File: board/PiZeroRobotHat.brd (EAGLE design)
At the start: 65 x 30 mm, 31 parts, among them IC1 TPS63061, IC2 MEGA8-AI, J1 AVRISP6_TP, Q1 CSTCR6M00G53Z, U1 DRV8835, U2 PCA9306, X1 1751248, X2 1751248, X3 1751248

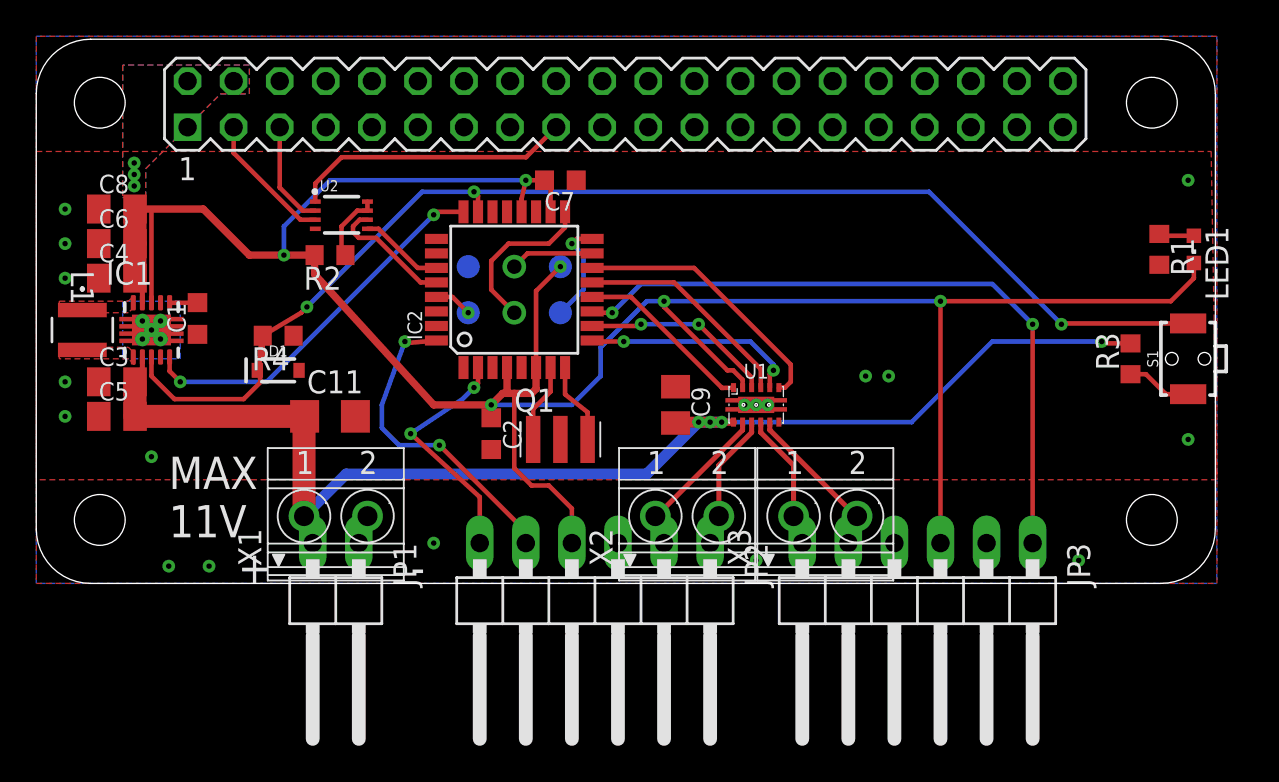
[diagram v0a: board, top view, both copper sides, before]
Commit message: board improvements
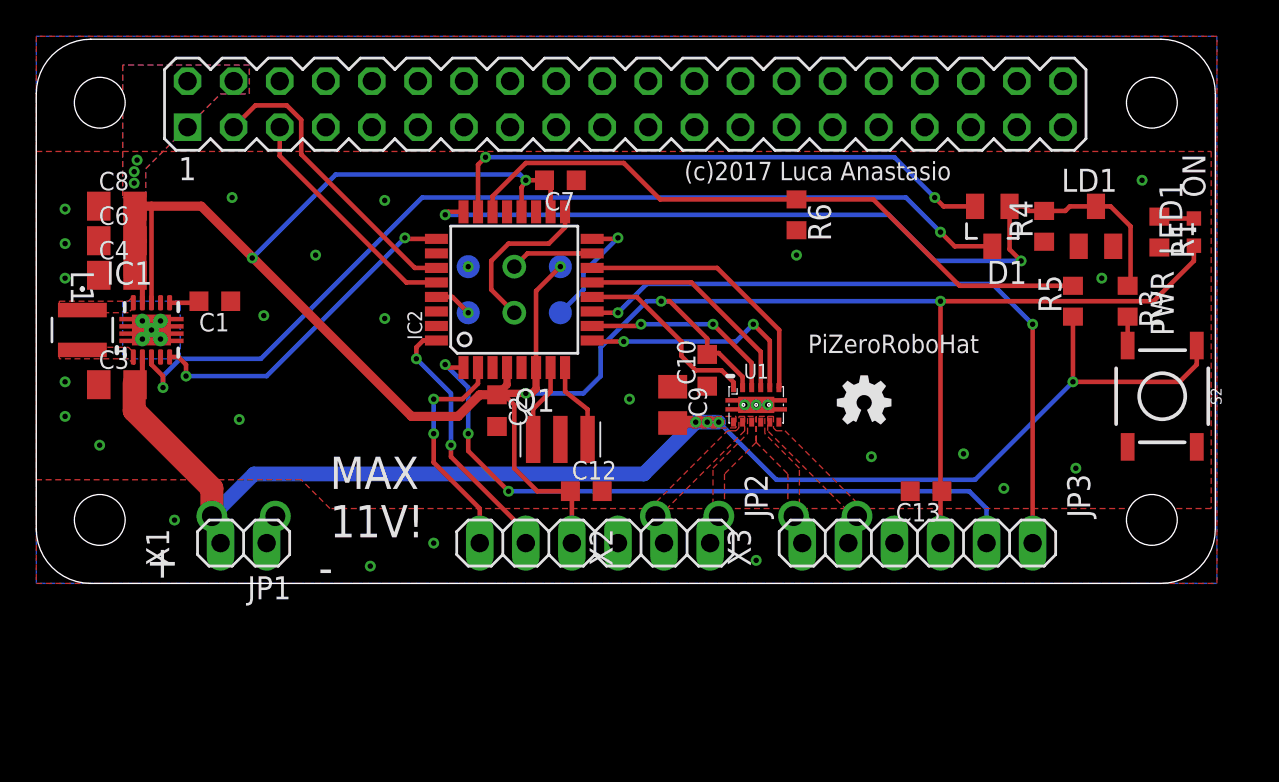
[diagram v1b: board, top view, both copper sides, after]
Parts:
- removed C11: 100uF, eagle-ltspice:C1206
- removed C5: 10uF, rcl:C0805K
- removed R2: 200K, resistor:R0603
- removed S1: MOMENTARY-SWITCH-SPST-SMD-RIGHT-ANGLE, SparkFun-Switches:TACTILE_SWITCH_SMD_RIGHT_ANGLE
- removed U2: PCA9306, SparkFun-IC-Comms:PCA9306DC
- added C10, C12, C13: 0.1uF, rcl:C0603K
- added LD1: PL006-WCR12, led:SOT23
- added R5: 470k, rcl:R0603
- added R6: 330k, rcl:R0603
- added S2: MOMENTARY-SWITCH-SPST-SMD-5.2-REDUNDANT, SparkFun-Switches:TACTILE_SWITCH_SMD_5.2MM
- D1: value 5.6V -> BAT54C; device SparkFun-DiscreteSemi:SOD-323 -> diode:SOT23
- JP1: device pinhead:1X02/90 -> pinhead:1X02
- JP2, JP3: device pinhead:1X06/90 -> pinhead:1X06
- R3: value 1M -> 10K
- R4: value 10M -> 1M
- moved R4 42.7 mm to (55.6, 19.7), turned to 90 degrees
- moved D1 40.2 mm to (52.7, 19.7), turned to 180 degrees
- moved JP1 6.35 mm to (11.4, 2.22)
- moved X1 5.08 mm to (11.4, 3.81)
- moved JP2 3.81 mm to (30.8, 2.22)
- moved JP3 3.81 mm to (48.6, 2.22)
- moved R3 3.18 mm to (60.2, 15.6), turned to 270 degrees
- moved C1 1.35 mm to (9.84, 15.6), turned to 180 degrees
- moved C2 1.31 mm to (25.4, 9.53)
- moved LED1 0.95 mm to (63.8, 19.4), turned to 0 degrees
- moved R1 0.95 mm to (61.9, 19.4)
- moved C3 0.16 mm to (4.45, 11.0)
- moved C8 0.16 mm to (4.45, 20.8)
- moved C4 0.16 mm to (4.45, 17.0)
- moved C6 0.16 mm to (4.45, 18.9)
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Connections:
- net N$10 renamed M1A
- net N$6 renamed M0A
- net N$8 renamed M1B
- net N$9 renamed M0B
- removed net 3.3V: U$1.17, U2.1
- removed net N$2: R2.1, U2.7, U2.8
- removed net SCL1: U$1.5, U2.2
- removed net SCL2: IC2.28, U2.6
- removed net SDA1: U$1.3, U2.3
- removed net SDA2: IC2.27, U2.5
- new net BUTTON: D1.1, IC2.24, LD1.3, R3.1, R4.2
- new net PS_ON: D1.2, IC2.23
- new net SCL: IC2.28, U$1.5
- new net SDA: IC2.27, U$1.3
- net 5V: now also C10.2, C12.1, C13.1, LED1.A; no longer LED1.C, R2.2
- net ENABLE: now also D1.3; no longer D1.C, IC2.23, R4.2, S1.2
- net GND: now also C10.1, C12.2, C13.2, LD1.1, R6.2; no longer C11.2, C5.1, D1.A, U2.4
- net N$1: now also R3.2, S2.3, S2.4; no longer R3.1, S1.1
- net N$7: now also LED1.C; no longer LED1.A
- net POWER_GOOD: now also IC2.25; no longer IC2.24
- net VBAT: now also R5.2, R6.1
- net VIN: now also R5.1, S2.1, S2.2; no longer C11.1, C5.2, R3.2
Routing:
- net BUTTON: track 0.00 -> 47.8 mm, vias 0 -> 2
- net ENC1_A: track 0.00 -> 38.2 mm, vias 0 -> 3
- net VBAT: track 0.00 -> 36.4 mm
- net PS_ON: track 0.00 -> 31.3 mm, vias 0 -> 2
- net ENABLE: track 71.8 -> 53.5 mm, vias 3 -> 2
- net SDA: track 0.00 -> 16.5 mm
- net 3.3V: track 15.6 -> 0.00 mm
- net SCL: track 0.00 -> 13.1 mm
- net VIN: track 71.1 -> 81.9 mm
- net SDA1: track 7.45 -> 0.00 mm
- net M1B: track 8.90 -> 1.69 mm
- net M0B: track 8.77 -> 1.56 mm
- net SCL2: track 7.01 -> 0.00 mm
- net M1A: track 7.62 -> 1.69 mm
- net M0A: track 7.62 -> 1.69 mm
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- added copper zone on layer 1, net M0A
- added copper zone on layer 1, net M0B
- added copper zone on layer 1, net M1A
- added copper zone on layer 1, net M1B
- added copper zone on layer 1, net VIN
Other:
- board text added: "(c)2017 Luca Anastasio"
- board text added: "/home/luca/Immagini/oshw.bmp"
- board text added: "MAX 11V!"
- board text added: "ON"
- board text added: "PWR"
- board text added: "PiZeroRoboHat"
- board text removed: "MAX 11V"

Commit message: board improvements
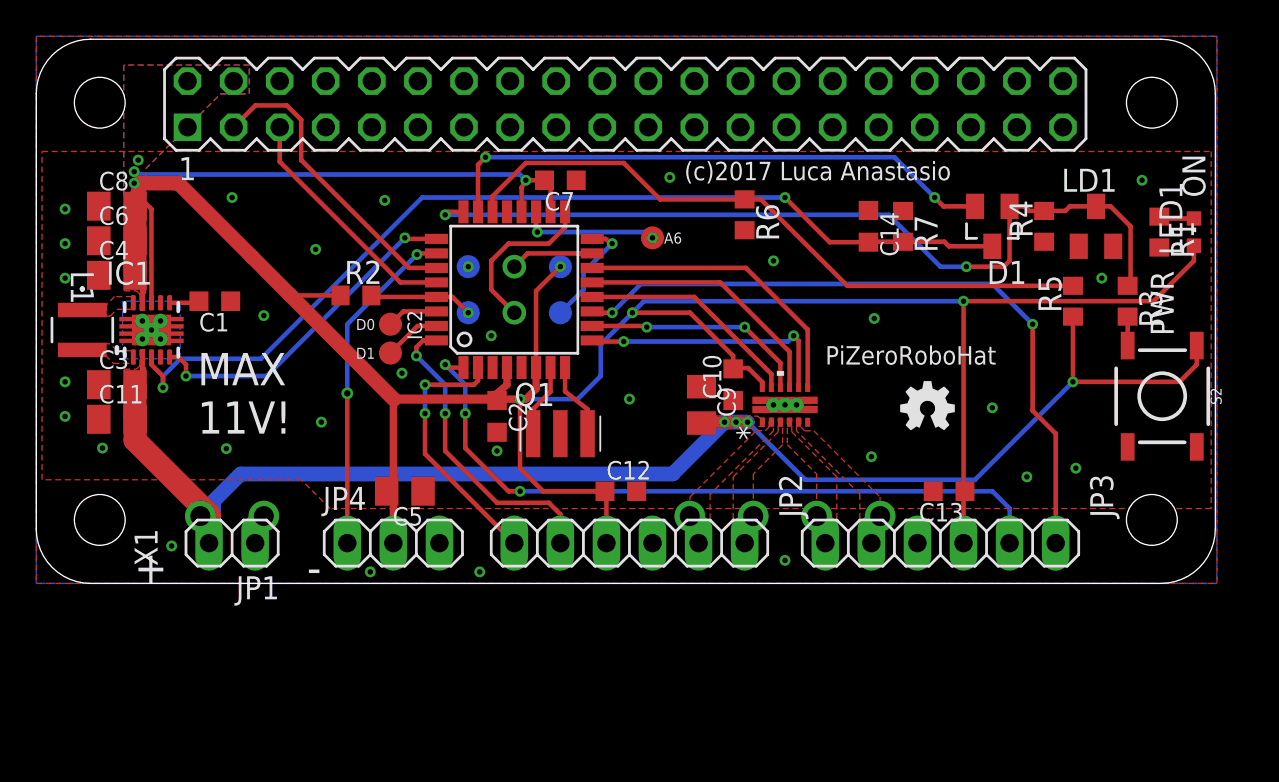
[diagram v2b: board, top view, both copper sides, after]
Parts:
- removed U1: DRV8835, bt_motordriver:WSON_2X3
- removed X2, X3: 1751248, con-phoenix-350:1751248
- added C11, C5: 10uF, rcl:C0805K
- added C14: 0.1uF, rcl:C0603K
- added JP4: (no value), pinhead:1X03
- added R2: 10K, resistor:R0603
- added R7: 1M, resistor:R0603
- added TP1, TP2, TP3: TEST-POINT3X5, SparkFun-Connectors:PAD.03X.05
- added U2: DRV8835DSSR, drv8835:DSS12_P9X2
- added X4: 1751264, con-phoenix-350:1751264
- moved R6 2.86 mm to (39.1, 20.3)
- moved C12 1.91 mm to (32.2, 5.08)
- moved JP2 1.91 mm to (32.7, 2.22)
- moved C10 1.63 mm to (38.4, 11.0)
- moved C9 1.59 mm to (36.7, 9.84)
- moved C13 1.27 mm to (50.3, 5.08)
- moved JP3 1.27 mm to (49.8, 2.22)
- moved JP1 0.63 mm to (10.8, 2.22)
- moved X1 0.63 mm to (10.8, 3.81)
- moved C2 0.32 mm to (25.4, 9.21)
- moved Q1 0.32 mm to (28.9, 8.26)
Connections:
- new net 0: IC2.30, TP1.P$1
- new net 1: IC2.31, TP2.P$1
- new net N$8: IC2.19, TP3.P$1
- new net SERVO: IC2.26, JP4.1
- net 5V: now also C5.2, JP4.2, R2.1, U2.12; no longer U1.11
- net ENABLE: now also C14.2, R7.2
- net EN_A: now also U2.9; no longer U1.9
- net EN_B: now also U2.7; no longer U1.7
- net GND: now also C11.1, C14.1, C5.1, JP4.3, R7.1, U2.13, U2.14, U2.15, U2.16, U2.17, U2.18, U2.6, U2.P$1, U2.P$2, U2.P$3; no longer U1.6, U1.PAD, U1.PAD1, U1.PAD2, U1.PAD3, U1.PAD4
- net M0A: now also U2.3, X4.2; no longer U1.3, X2.2
- net M0B: now also U2.2, X4.1; no longer U1.2, X2.1
- net M1A: now also U2.4, X4.3; no longer U1.4, X3.1
- net M1B: now also U2.5, X4.4; no longer U1.5, X3.2
- net MODE: now also U2.11; no longer U1.12
- net PH_A: now also U2.10; no longer U1.10
- net PH_B: now also U2.8; no longer U1.8
- net RST: now also R2.2
- net VIN: now also C11.2, U2.1; no longer U1.1
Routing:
- net 5V: track 143.7 -> 167.3 mm, vias 9 -> 8
- net SERVO: track 0.00 -> 18.6 mm, vias 0 -> 2
- net N$8: track 0.00 -> 7.63 mm, vias 0 -> 2
- net RST: track 2.11 -> 6.19 mm
- net 1: track 0.00 -> 3.15 mm
- net VIN: track 81.9 -> 85.0 mm
- net 0: track 0.00 -> 2.83 mm
- net ENC0_A: track 14.6 -> 17.0 mm
- net MODE: track 10.5 -> 12.4 mm
- net ENC0_B: track 12.7 -> 14.5 mm
- net EN_A: track 12.9 -> 14.4 mm
- net M0B: track 1.56 -> 0.00 mm
- net EN_B: track 14.9 -> 16.5 mm
- net PH_A: track 11.1 -> 12.6 mm
- net ENC1_A: track 38.2 -> 39.4 mm
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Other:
- board text added: "5V"
- board text added: "A"
- board text added: "A6"
- board text added: "B"
- board text added: "D0"
- board text added: "D1"
- board text added: "M+"
- board text added: "M-"
- board text added: "S"
- board text removed: "/home/luca/Immagini/oshw.bmp"

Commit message: board improvements
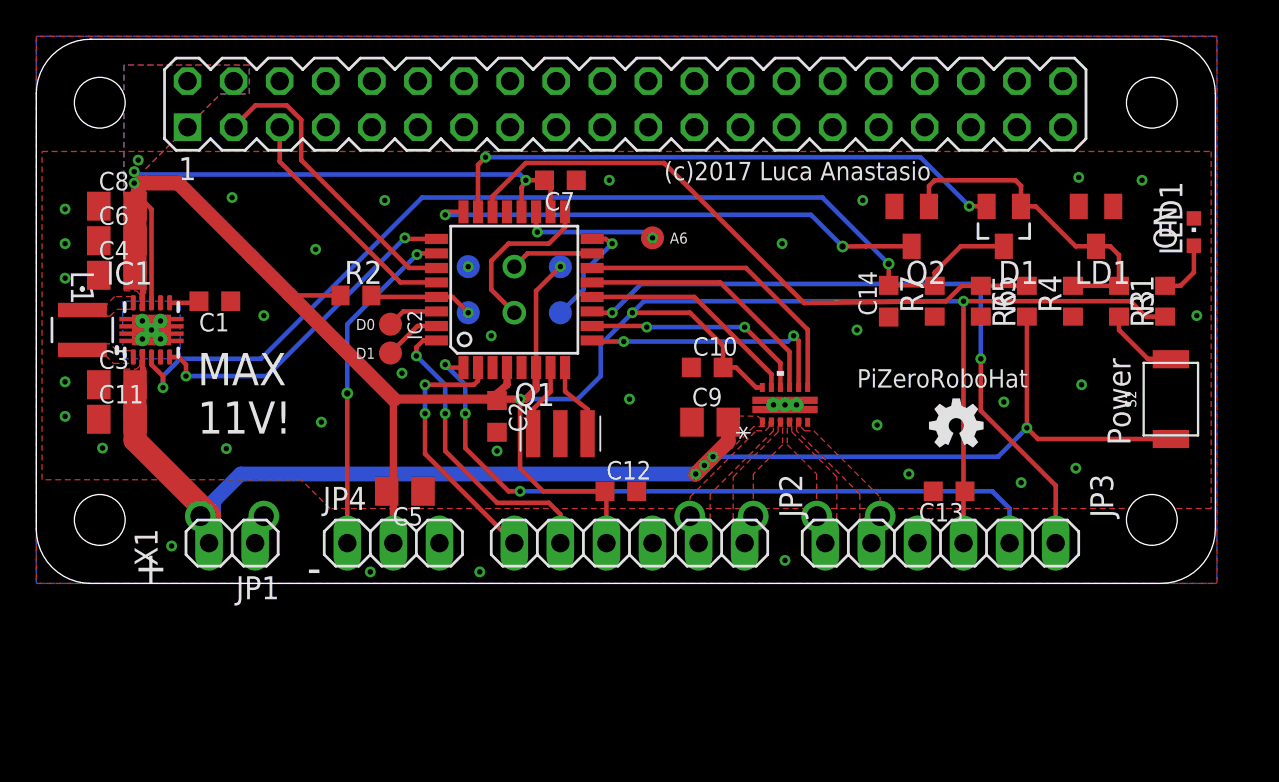
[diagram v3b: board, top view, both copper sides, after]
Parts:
- added Q2: (no value), adafruit:SOT23
- R3: value 10K -> 1K
- R4, R7: value 1M -> 100K
- S2: value MOMENTARY-SWITCH-SPST-SMD-5.2-REDUNDANT -> MOMENTARY-SWITCH-SPST; device SparkFun-Switches:TACTILE_SWITCH_SMD_5.2MM -> SparkFun-Switches:TACTILE_SWITCH_SMD_4X3MM
- moved R6 13.9 mm to (52.1, 15.6)
- moved R7 4.48 mm to (49.5, 15.6), turned to 90 degrees
- moved R4 4.42 mm to (57.1, 15.6)
- moved C14 4.27 mm to (47.0, 15.6), turned to 90 degrees
- moved R1 3.82 mm to (62.2, 15.6), turned to 90 degrees
- moved R5 2.54 mm to (54.6, 15.6)
- moved C10 1.72 mm to (37.0, 11.9), turned to 0 degrees
- moved C9 1.06 mm to (37.1, 8.89), turned to 0 degrees
- moved D1 0.64 mm to (53.3, 19.7)
- moved S2 0.50 mm to (62.5, 10.2), turned to 90 degrees
- moved R3 0.48 mm to (59.7, 15.6)
- turned LD1 to 180 degrees
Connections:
- removed net N$7: LED1.C, R1.1
- new net BT: D1.1, LD1.3, Q2.1, R3.1, R4.2
- new net N$2: LED1.A, R1.2
- net 5V: now also R1.1; no longer LED1.A
- net BUTTON: now also Q2.3; no longer D1.1, LD1.3, R3.1, R4.2
- net GND: now also LED1.C, Q2.2; no longer R1.2
- net N$1: now also S2.2; no longer S2.3, S2.4
- net VIN: no longer S2.2
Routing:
- net BUTTON: track 47.2 -> 27.5 mm
- net BT: track 0.00 -> 18.3 mm
- net ENABLE: track 53.5 -> 57.1 mm
- net N$2: track 0.00 -> 3.37 mm
- net 5V: track 167.3 -> 164.4 mm
- net VIN: track 85.0 -> 82.1 mm
- net N$1: track 1.59 -> 4.25 mm
- net N$7: track 1.95 -> 0.00 mm
- net VBAT: track 36.4 -> 34.6 mm
- net ENC1_B: track 38.5 -> 37.8 mm
- net PS_ON: track 31.3 -> 31.9 mm
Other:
- board text added: "Power"
- board text removed: "PWR"
